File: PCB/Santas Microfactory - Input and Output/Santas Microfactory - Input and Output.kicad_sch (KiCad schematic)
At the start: 0 parts

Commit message: Update Input Output Board
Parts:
- added D1, D10, D11, D12, D13, D14, D15, D16, D17, D18, D19, D2, D20, D21, D22, D23, D24, D25, D26, D27, D28, D29, D3, D30, D31, D32, D33, D34, D35, D36, D37, D38, D39, D4, D40, D41, D42, D43, D44, D45, D46, D47, D48, D49, D5, D50, D51, D52, D53, D54, D55, D56, D57, D58, D59, D6, D60, D61, D62, D63, D64, D65, D66, D67, D68, D69, D7, D70, D71, D72, D73, D74, D75, D76, D77, D8, D9: LED, LED_THT:LED_Rectangular_W5.0mm_H2.0mm, symbol Device:LED
- added H1, H2, H3, H4: MountingHole, MountingHole:MountingHole_3.2mm_M3_Pad_Via, symbol Mechanical:MountingHole
- added J1: Conn_01x04_Pin, Connector_PinHeader_2.54mm:PinHeader_1x04_P2.54mm_Vertical, symbol Connector:Conn_01x04_Pin
- added J10: Conn_01x14_Pin, Connector_PinHeader_2.54mm:PinHeader_1x14_P2.54mm_Vertical, symbol Connector:Conn_01x14_Pin
- added J2: Conn_01x08_Pin, Connector_PinHeader_2.54mm:PinHeader_1x08_P2.54mm_Vertical, symbol Connector:Conn_01x08_Pin
- added J3, J4, J5, J6, J8, J9: Conn_01x10_Pin, Connector_PinHeader_2.54mm:PinHeader_1x10_P2.54mm_Vertical, symbol Connector:Conn_01x10_Pin
- added J7: Conn_01x06_Pin, Connector_PinHeader_2.54mm:PinHeader_1x06_P2.54mm_Vertical, symbol Connector:Conn_01x06_Pin
- added R1, R10, R11, R12, R13, R14, R15, R16, R17, R18, R19, R2, R20, R21, R22, R23, R24, R25, R26, R27, R28, R29, R3, R30, R31, R32, R33, R34, R35, R36, R37, R38, R39, R4, R40, R41, R42, R43, R44, R45, R46, R47, R48, R49, R5, R50, R51, R52, R53, R54, R55, R56, R57, R58, R59, R6, R60, R61, R62, R63, R64, R65, R66, R67, R68, R69, R7, R70, R71, R72, R73, R74, R75, R76, R77, R8, R9: 330, Resistor_THT:R_Axial_DIN0207_L6.3mm_D2.5mm_P10.16mm_Horizontal, symbol Device:R
- added SW1, SW10, SW11, SW2, SW3, SW4, SW5, SW6, SW7, SW8, SW9: SW_DPDT_x2, imported_components_other:SW-TH_MT-0-103-A101-M200-RS, symbol Switch:SW_DPDT_x2
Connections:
- new net: D36.2 (A), R36.1
- new net: D40.2 (A), R40.1
- new net: D69.2 (A), R69.1
- new net: D50.2 (A), R50.1
- new net: D20.2 (A), R20.1
- new net: D6.2 (A), R6.1
- new net: D70.2 (A), R70.1
- new net: D3.2 (A), R3.1
- new net: D49.2 (A), R49.1
- new net: D35.2 (A), R35.1
- new net: D63.2 (A), R63.1
- new net: D38.2 (A), R38.1
- new net: D46.2 (A), R46.1
- new net: D56.2 (A), R56.1
- new net: D54.2 (A), R54.1
- new net: D9.2 (A), R9.1
- new net: D65.2 (A), R65.1
- new net: D48.2 (A), R48.1
- new net: D73.2 (A), R73.1
- new net: D19.2 (A), R19.1
- new net: D75.2 (A), R75.1
- new net: D11.2 (A), R11.1
- new net: D29.2 (A), R29.1
- new net: D59.2 (A), R59.1
- new net: D14.2 (A), R14.1
- new net: D67.2 (A), R67.1
- new net: D1.2 (A), R1.1
- new net: D17.2 (A), R17.1
- new net: D66.2 (A), R66.1
- new net: D58.2 (A), R58.1
- new net: D21.2 (A), R21.1
- new net: D47.2 (A), R47.1
- new net: D16.2 (A), R16.1
- new net: D77.2 (A), R77.1
- new net: D25.2 (A), R25.1
- new net: D74.2 (A), R74.1
- new net: D12.2 (A), R12.1
- new net: D37.2 (A), R37.1
- new net: D32.2 (A), R32.1
- new net: D5.2 (A), R5.1
- new net: D53.2 (A), R53.1
- new net: D76.2 (A), R76.1
- new net: D7.2 (A), R7.1
- new net: D41.2 (A), R41.1
- new net: D18.2 (A), R18.1
- new net: D22.2 (A), R22.1
- new net: D39.2 (A), R39.1
- new net: D30.2 (A), R30.1
- new net: D15.2 (A), R15.1
- new net: D23.2 (A), R23.1
- new net: D71.2 (A), R71.1
- new net: D27.2 (A), R27.1
- new net: D24.2 (A), R24.1
- new net: D26.2 (A), R26.1
- new net: D57.2 (A), R57.1
- new net: D60.2 (A), R60.1
- new net: D61.2 (A), R61.1
- new net: D33.2 (A), R33.1
- new net: D8.2 (A), R8.1
- new net: D51.2 (A), R51.1
- new net: D42.2 (A), R42.1
- new net: D34.2 (A), R34.1
- new net: D52.2 (A), R52.1
- new net: D10.2 (A), R10.1
- new net: D43.2 (A), R43.1
- new net: D55.2 (A), R55.1
- new net: D28.2 (A), R28.1
- new net: D62.2 (A), R62.1
- new net: D2.2 (A), R2.1
- new net: D68.2 (A), R68.1
- new net: D45.2 (A), R45.1
- new net: D64.2 (A), R64.1
- new net: D4.2 (A), R4.1
- new net: D31.2 (A), R31.1
- new net: D44.2 (A), R44.1
- new net: D13.2 (A), R13.1
- new net: D72.2 (A), R72.1
- new net +5V: J10.1 (Pin_1), SW1.1 (A), SW10.1 (A), SW11.1 (A), SW2.1 (A), SW3.1 (A), SW4.1 (A), SW5.1 (A), SW6.1 (A), SW7.1 (A), SW8.1 (A), SW9.1 (A)
- new net CLK: J10.13 (Pin_13), R1.2
- new net GND: D1.1 (K), D10.1 (K), D11.1 (K), D12.1 (K), D13.1 (K), D14.1 (K), D15.1 (K), D16.1 (K), D17.1 (K), D18.1 (K), D19.1 (K), D2.1 (K), D20.1 (K), D21.1 (K), D22.1 (K), D23.1 (K), D24.1 (K), D25.1 (K), D26.1 (K), D27.1 (K), D28.1 (K), D29.1 (K), D3.1 (K), D30.1 (K), D31.1 (K), D32.1 (K), D33.1 (K), D34.1 (K), D35.1 (K), D36.1 (K), D37.1 (K), D38.1 (K), D39.1 (K), D4.1 (K), D40.1 (K), D41.1 (K), D42.1 (K), D43.1 (K), D44.1 (K), D45.1 (K), D46.1 (K), D47.1 (K), D48.1 (K), D49.1 (K), D5.1 (K), D50.1 (K), D51.1 (K), D52.1 (K), D53.1 (K), D54.1 (K), D55.1 (K), D56.1 (K), D57.1 (K), D58.1 (K), D59.1 (K), D6.1 (K), D60.1 (K), D61.1 (K), D62.1 (K), D63.1 (K), D64.1 (K), D65.1 (K), D66.1 (K), D67.1 (K), D68.1 (K), D69.1 (K), D7.1 (K), D70.1 (K), D71.1 (K), D72.1 (K), D73.1 (K), D74.1 (K), D75.1 (K), D76.1 (K), D77.1 (K), D8.1 (K), D9.1 (K), J3.10 (Pin_10), J4.10 (Pin_10), J5.10 (Pin_10), J6.10 (Pin_10), SW1.3 (C), SW10.3 (C), SW11.3 (C), SW2.3 (C), SW3.3 (C), SW4.3 (C), SW5.3 (C), SW6.3 (C), SW7.3 (C), SW8.3 (C), SW9.3 (C)
- new net HALT: J10.14 (Pin_14), R2.2
- new net HEART0: J1.1 (Pin_1), R67.2
- new net HEART1: J1.2 (Pin_2), R68.2
- new net HEART2: J1.3 (Pin_3), R69.2
- new net HEART3: J1.4 (Pin_4), R70.2
- new net INPUT0: J10.6 (Pin_6), SW3.2 (B)
- new net INPUT1: J10.7 (Pin_7), SW5.2 (B)
- new net INPUT2: J10.8 (Pin_8), SW7.2 (B)
- new net INPUT3: J10.9 (Pin_9), SW9.2 (B)
- new net INPUT4: J10.10 (Pin_10), SW10.2 (B)
- new net INPUT5: J10.11 (Pin_11), SW11.2 (B)
- new net LOAD0: J7.1 (Pin_1), R71.2
- new net LOAD1: J7.2 (Pin_2), R72.2
- new net LOAD2: J7.3 (Pin_3), R73.2
- new net LOAD3: J7.4 (Pin_4), R74.2
- new net LOAD4: J7.5 (Pin_5), R75.2
- new net LOAD5: J7.6 (Pin_6), R76.2
- new net OUT_C0: J8.1 (Pin_1), R49.2
- new net OUT_C1: J8.2 (Pin_2), R50.2
- new net OUT_C2: R51.2
- new net OUT_C3: R52.2
- new net OUT_C4: J8.5 (Pin_5), R53.2
- new net OUT_C5: R54.2
- new net OUT_C6: R55.2
- new net OUT_C7: J8.8 (Pin_8), R56.2
- new net OUT_C8: R57.2
- new net OUT_C9: R58.2
- new net OUT_G0: J9.1 (Pin_1), R39.2
- new net OUT_G1: J9.2 (Pin_2), R40.2
- new net OUT_G2: R41.2
- new net OUT_G3: R42.2
- new net OUT_G4: J9.5 (Pin_5), R43.2
- new net OUT_G5: R44.2
- new net OUT_G6: R45.2
- new net OUT_G7: J9.8 (Pin_8), R46.2
- new net OUT_G8: R47.2
- new net OUT_G9: R48.2
- new net OUT_H0: J2.8 (Pin_8), R59.2
- new net OUT_H1: J2.7 (Pin_7), R60.2
- new net OUT_H2: J2.6 (Pin_6), R61.2
- new net OUT_H3: J2.5 (Pin_5), R62.2
- new net OUT_H4: J2.4 (Pin_4), R63.2
- new net OUT_H5: J2.3 (Pin_3), R64.2
- new net OUT_H6: J2.2 (Pin_2), R65.2
- new net OUT_H7: J2.1 (Pin_1), R66.2
- new net RESET: J10.12 (Pin_12), R77.2, SW1.2 (B)
- new net S0_C0: J4.9 (Pin_9), R9.2
- new net S0_C1: J4.6 (Pin_6), R10.2
- new net S0_C2: J4.3 (Pin_3), R11.2
- new net S0_C3: J6.9 (Pin_9), R12.2
- new net S0_C4: J6.6 (Pin_6), R13.2
- new net S0_C5: J6.3 (Pin_3), R14.2
- new net S0_G0: J3.9 (Pin_9), R3.2
- new net S0_G1: J3.6 (Pin_6), R4.2
- new net S0_G2: J3.3 (Pin_3), R5.2
- new net S0_G3: J5.9 (Pin_9), R6.2
- new net S0_G4: J5.6 (Pin_6), R7.2
- new net S0_G5: J5.3 (Pin_3), R8.2
- new net S1_C0: J4.8 (Pin_8), R21.2
- new net S1_C1: J4.5 (Pin_5), R22.2
- new net S1_C2: J4.2 (Pin_2), R23.2
- new net S1_C3: J6.8 (Pin_8), R24.2
- new net S1_C4: J6.5 (Pin_5), R25.2
- new net S1_C5: J6.2 (Pin_2), R26.2
- new net S1_G0: J3.8 (Pin_8), R15.2
- new net S1_G1: J3.5 (Pin_5), R16.2
- new net S1_G2: J3.2 (Pin_2), R17.2
- new net S1_G3: J5.8 (Pin_8), R18.2
- new net S1_G4: J5.5 (Pin_5), R19.2
- new net S1_G5: J5.2 (Pin_2), R20.2
- new net S2_C0: J4.7 (Pin_7), R33.2
- new net S2_C1: J4.4 (Pin_4), R34.2
- new net S2_C2: J4.1 (Pin_1), R35.2
- new net S2_C3: J6.7 (Pin_7), R36.2
- new net S2_C4: J6.4 (Pin_4), R37.2
- new net S2_C5: J6.1 (Pin_1), R38.2
- new net S2_G0: J3.7 (Pin_7), R27.2
- new net S2_G1: J3.4 (Pin_4), R28.2
- new net S2_G2: J3.1 (Pin_1), R29.2
- new net S2_G3: J5.7 (Pin_7), R30.2
- new net S2_G4: J5.4 (Pin_4), R31.2
- new net S2_G5: J5.1 (Pin_1), R32.2
- new net SEED_1: J10.2 (Pin_2), SW2.2 (B)
- new net SEED_2: J10.3 (Pin_3), SW4.2 (B)
- new net SEED_3: J10.4 (Pin_4), SW6.2 (B)
- new net SEED_4: J10.5 (Pin_5), SW8.2 (B)
- new net TAP_C2: J8.3 (Pin_3)
- new net TAP_C3: J8.4 (Pin_4)
- new net TAP_C5: J8.6 (Pin_6)
- new net TAP_C6: J8.7 (Pin_7)
- new net TAP_C8: J8.9 (Pin_9)
- new net TAP_C9: J8.10 (Pin_10)
- new net TAP_G2: J9.3 (Pin_3)
- new net TAP_G3: J9.4 (Pin_4)
- new net TAP_G5: J9.6 (Pin_6)
- new net TAP_G6: J9.7 (Pin_7)
- new net TAP_G8: J9.9 (Pin_9)
- new net TAP_G9: J9.10 (Pin_10)
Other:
- note added: "COAL CONVEYOR"
- note added: "GIFT CONVEYOR"
- note added: "HEALTH"
- note added: "INPUTS"
- note added: "MISC"
- note added: "SCORE"
- note added: "SCORING CHUTES"
- title: (none) -> Santas Microfactory - Input and Output

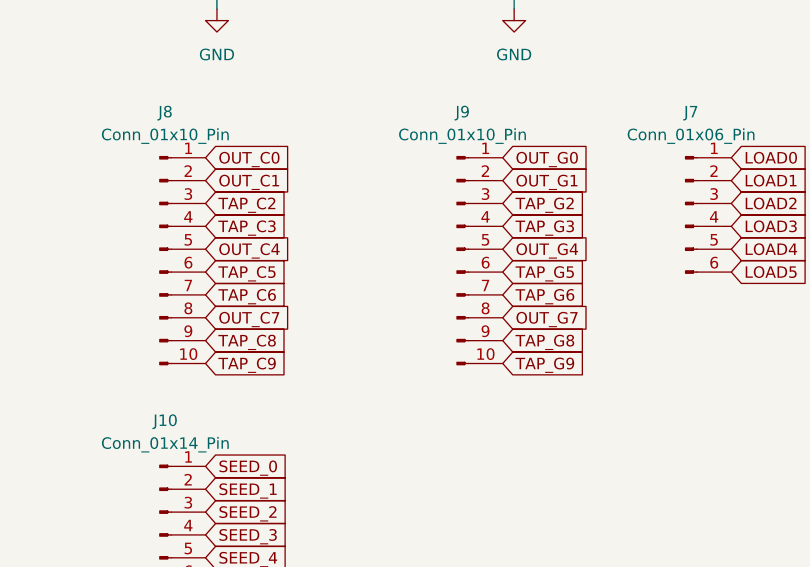
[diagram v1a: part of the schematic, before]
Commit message: Input Output Board Finished
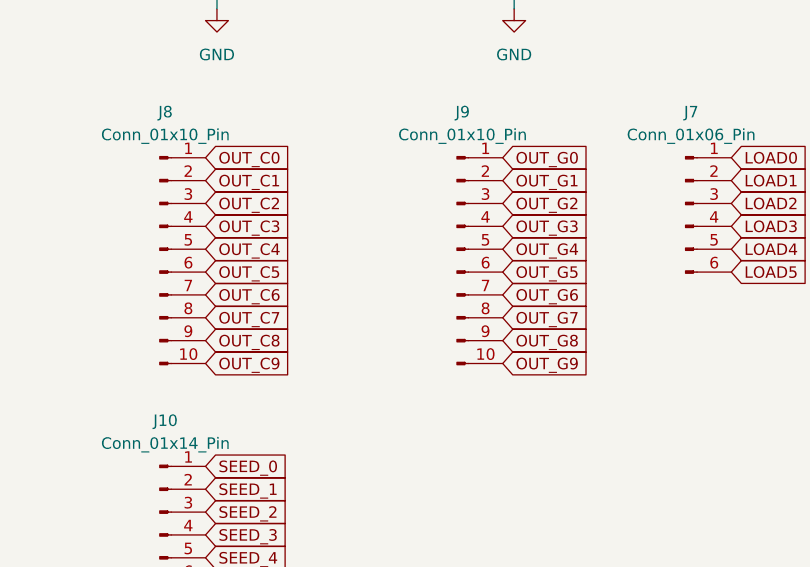
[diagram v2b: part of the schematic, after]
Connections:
- net TAP_C2 is gone; now on net OUT_C2: J8.3 (Pin_3)
- net TAP_C3 is gone; now on net OUT_C3: J8.4 (Pin_4)
- net TAP_C5 is gone; now on net OUT_C5: J8.6 (Pin_6)
- net TAP_C6 is gone; now on net OUT_C6: J8.7 (Pin_7)
- net TAP_C8 is gone; now on net OUT_C8: J8.9 (Pin_9)
- net TAP_C9 is gone; now on net OUT_C9: J8.10 (Pin_10)
- net TAP_G2 is gone; now on net OUT_G2: J9.3 (Pin_3)
- net TAP_G3 is gone; now on net OUT_G3: J9.4 (Pin_4)
- net TAP_G5 is gone; now on net OUT_G5: J9.6 (Pin_6)
- net TAP_G6 is gone; now on net OUT_G6: J9.7 (Pin_7)
- net TAP_G8 is gone; now on net OUT_G8: J9.9 (Pin_9)
- net TAP_G9 is gone; now on net OUT_G9: J9.10 (Pin_10)
